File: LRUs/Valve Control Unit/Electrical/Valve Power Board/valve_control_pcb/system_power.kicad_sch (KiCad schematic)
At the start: 49 parts, among them J10 Conn_01x02_Pin, J11 01x02_PinHeader, U14 TPS62933P, U15 TPS2116DRL, U16 TPS22810DBV, U17 AMS1117-3.3, U18 TPS22810DBV

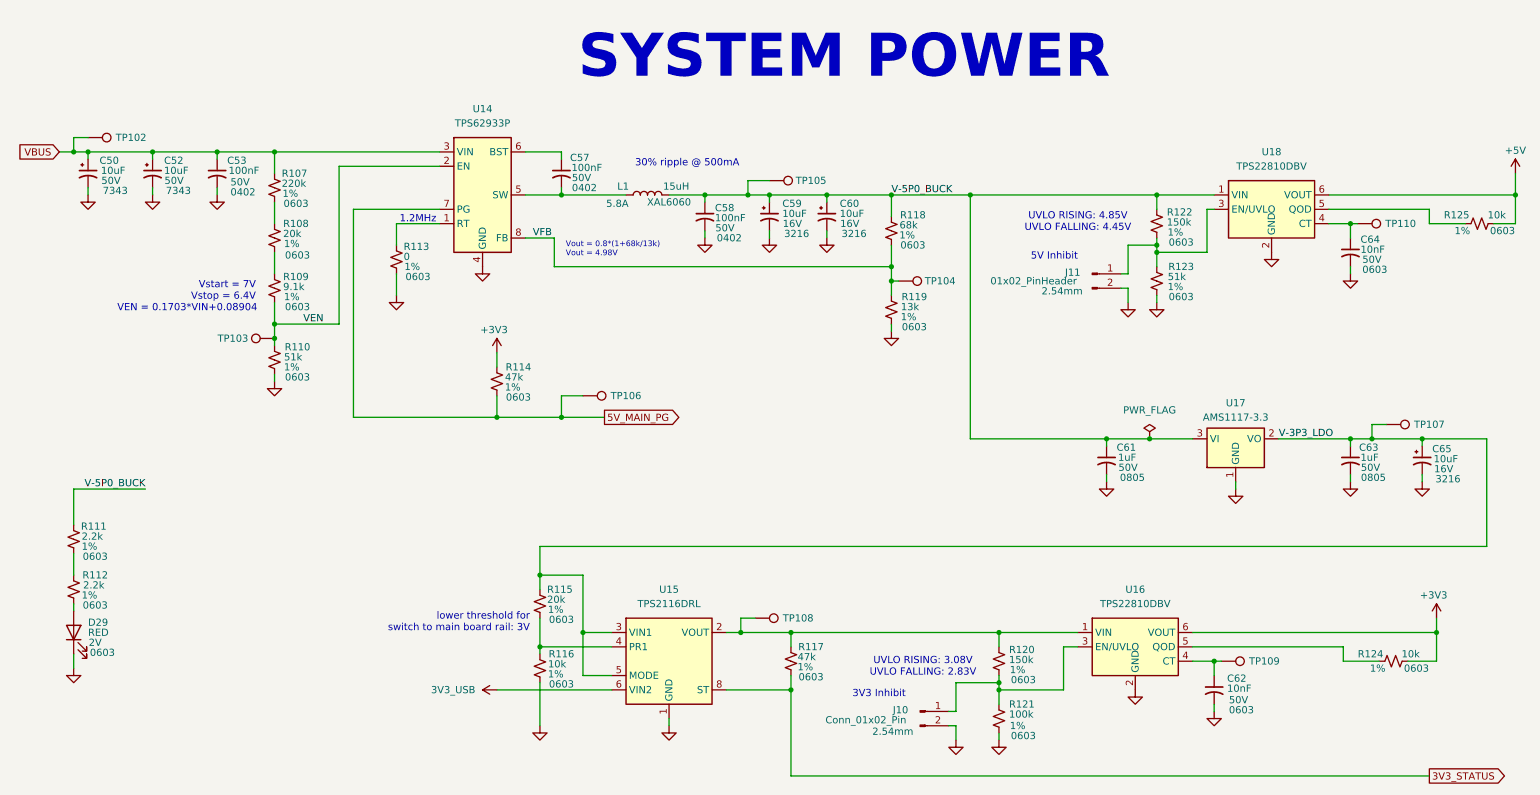
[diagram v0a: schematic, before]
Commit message: Commit da changes
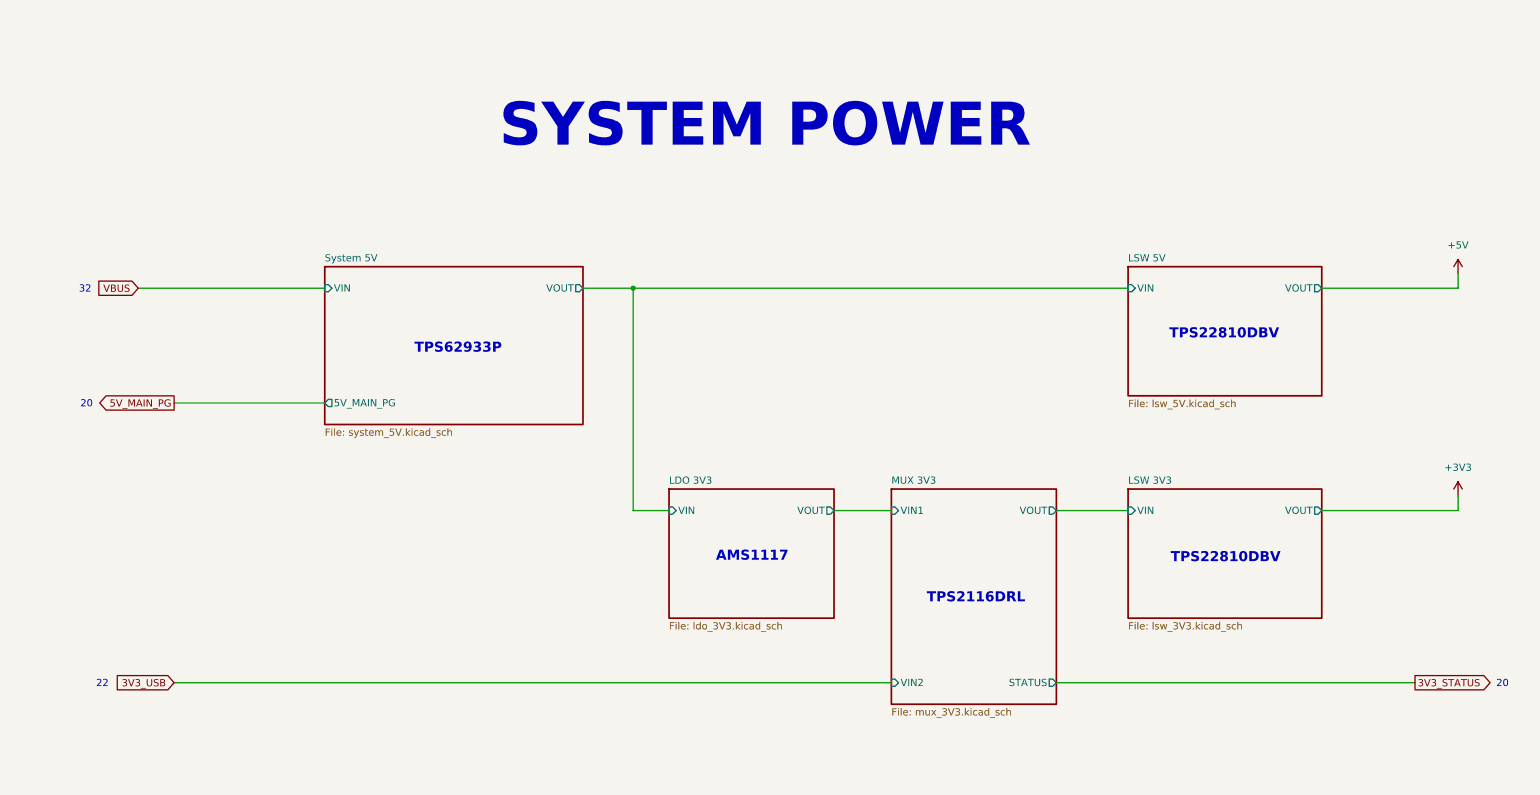
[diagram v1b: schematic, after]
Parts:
- removed C50, C52: 10uF, Capacitor_Tantalum_SMD:CP_EIA-7343-31_Kemet-D, symbol Device:C_Polarized_Small_US
- removed C53, C57, C58: 100nF, Capacitor_SMD:C_0402_1005Metric, symbol Device:C_Small_US
- removed C59, C60, C65: 10uF, Capacitor_Tantalum_SMD:CP_EIA-3216-18_Kemet-A, symbol Device:C_Polarized_Small_US
- removed C61, C63: 1uF, Capacitor_SMD:C_0805_2012Metric, symbol Device:C_Small_US
- removed C62, C64: 10nF, Capacitor_SMD:C_0603_1608Metric, symbol Device:C_Small_US
- removed D29: RED, LED_SMD:LED_0603_1608Metric, symbol Device:LED
- removed J10: Conn_01x02_Pin, Connector_PinHeader_2.54mm:PinHeader_1x02_P2.54mm_Vertical, symbol Connector:Conn_01x02_Pin
- removed J11: 01x02_PinHeader, Connector_PinHeader_2.54mm:PinHeader_1x02_P2.54mm_Vertical, symbol Connector:Conn_01x02_Pin
- removed L1: 15uH, Inductor_SMD:L_Coilcraft_XAL6060-XXX, symbol Device:L
- removed R107: 220k, Resistor_SMD:R_0603_1608Metric, symbol Device:R_Small_US
- removed R108, R115: 20k, Resistor_SMD:R_0603_1608Metric, symbol Device:R_Small_US
- removed R109: 9.1k, Resistor_SMD:R_0603_1608Metric, symbol Device:R_Small_US
- removed R110, R123: 51k, Resistor_SMD:R_0603_1608Metric, symbol Device:R_Small_US
- removed R111, R112: 2.2k, Resistor_SMD:R_0603_1608Metric, symbol Device:R_Small_US
- removed R113: 0, Resistor_SMD:R_0603_1608Metric, symbol Device:R_Small_US
- removed R114, R117: 47k, Resistor_SMD:R_0603_1608Metric, symbol Device:R_Small_US
- removed R116, R124, R125: 10k, Resistor_SMD:R_0603_1608Metric, symbol Device:R_Small_US
- removed R118: 68k, Resistor_SMD:R_0603_1608Metric, symbol Device:R_Small_US
- removed R119: 13k, Resistor_SMD:R_0603_1608Metric, symbol Device:R_Small_US
- removed R120, R122: 150k, Resistor_SMD:R_0603_1608Metric, symbol Device:R_Small_US
- removed R121: 100k, Resistor_SMD:R_0603_1608Metric, symbol Device:R_Small_US
- removed TP102, TP103, TP104, TP105, TP106, TP107, TP108, TP109, TP110: TestPoint, TestPoint:TestPoint_Pad_D2.0mm, symbol Connector:TestPoint
- removed U14: TPS62933P, Package_TO_SOT_SMD:SOT-583-8, symbol Regulator_Switching:TPS62933P
- removed U15: TPS2116DRL, Package_TO_SOT_SMD:SOT-583-8, symbol Power_Management:TPS2116DRL
- removed U16, U18: TPS22810DBV, Package_TO_SOT_SMD:SOT-23-6, symbol Power_Management:TPS22810DBV
- removed U17: AMS1117-3.3, Package_TO_SOT_SMD:SOT-223-3_TabPin2, symbol Regulator_Linear:AMS1117-3.3
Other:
- added sheet LDO 3V3 (ldo_3V3.kicad_sch)
- added sheet LSW 3V3 (lsw_3V3.kicad_sch)
- added sheet LSW 5V (lsw_5V.kicad_sch)
- added sheet MUX 3V3 (mux_3V3.kicad_sch)
- added sheet System 5V (system_5V.kicad_sch)
- note added: "20"
- note added: "22"
- note added: "32"
- note added: "AMS1117"
- note added: "TPS2116DRL"
- note added: "TPS22810DBV"
- note added: "TPS62933P"
- note removed: "1.2MHz"
- note removed: "30% ripple @ 500mA"
- note removed: "3V3 Inhibit"
- note removed: "5V Inhibit"
- note removed: "UVLO RISING: 3.08V UVLO FALLING: 2.83V"
- note removed: "UVLO RISING: 4.85V UVLO FALLING: 4.45V"
- note removed: "VEN = 0.1703*VIN+0.08904"
- note removed: "Vout = 0.8*(1+68k/13k) Vout = 4.98V"
- note removed: "Vstart = 7V Vstop = 6.4V"
- note removed: "lower threshold for switch to main board rail: 3V"
